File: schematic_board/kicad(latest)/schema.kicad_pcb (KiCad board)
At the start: 2 copper layers, 45 x 20 mm, 29 parts, among them IC1 TLC271CPS, IC2 LM311D, Q1 IRLML6244TRPBF

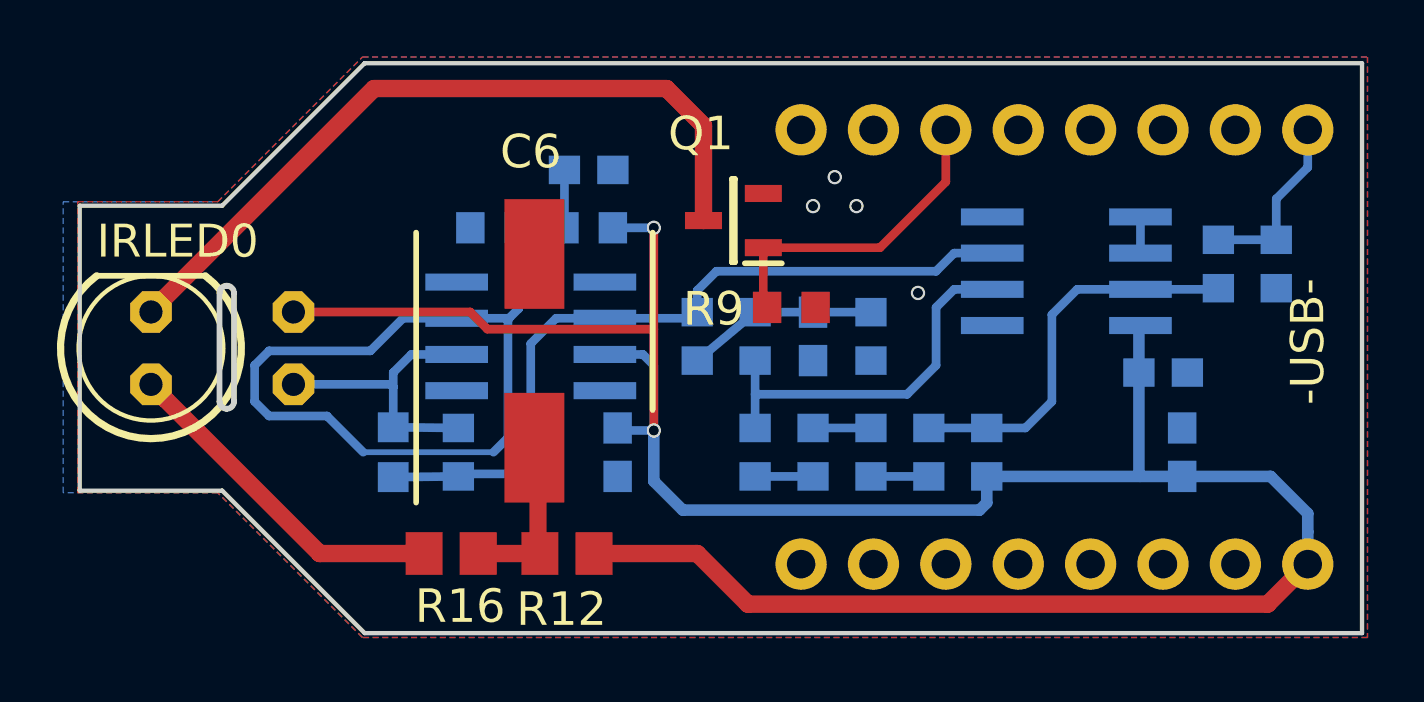
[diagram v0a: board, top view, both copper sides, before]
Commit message: Latest schematic and board design
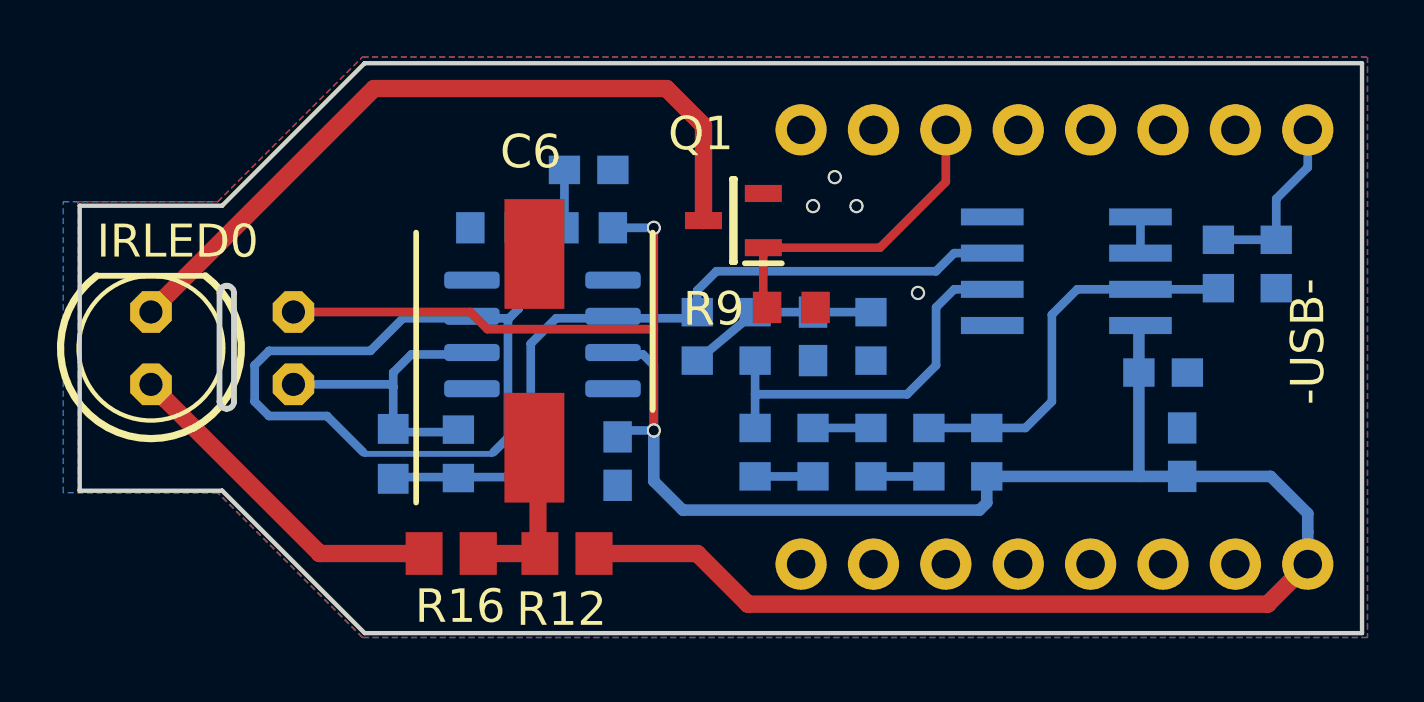
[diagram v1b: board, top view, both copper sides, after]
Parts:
- IC1: footprint schema:SO08_262 -> Package_SO:SOIC-8_3.9x4.9mm_P1.27mm
- moved IC1 0.42 mm to (142.2, 104.5), turned to 0 degrees
- moved C4 0.31 mm to (144.9, 109.0)
- moved C2 0.06 mm to (137.0, 108.7)
- moved R5 0.06 mm to (139.3, 108.7)
